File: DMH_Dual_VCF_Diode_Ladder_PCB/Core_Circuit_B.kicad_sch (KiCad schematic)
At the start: 41 parts, among them SW4 SW_SPDT, SW5 SW_SPDT, SW6 SW_SPDT, U4 TL074, U6 TL074

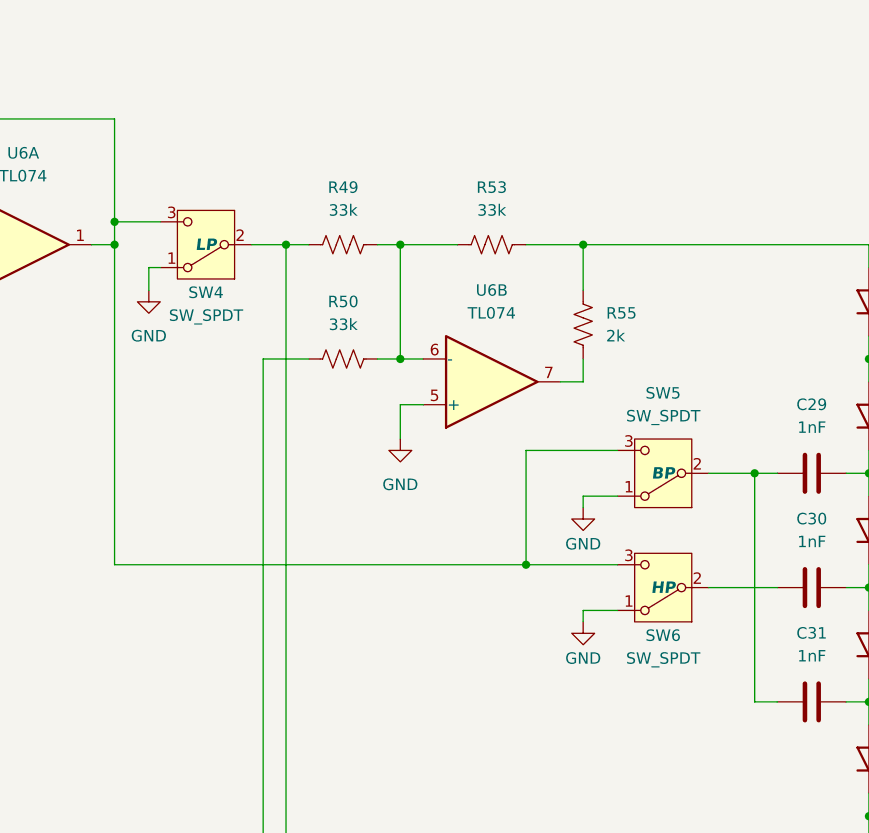
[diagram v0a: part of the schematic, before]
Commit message: Finished routing
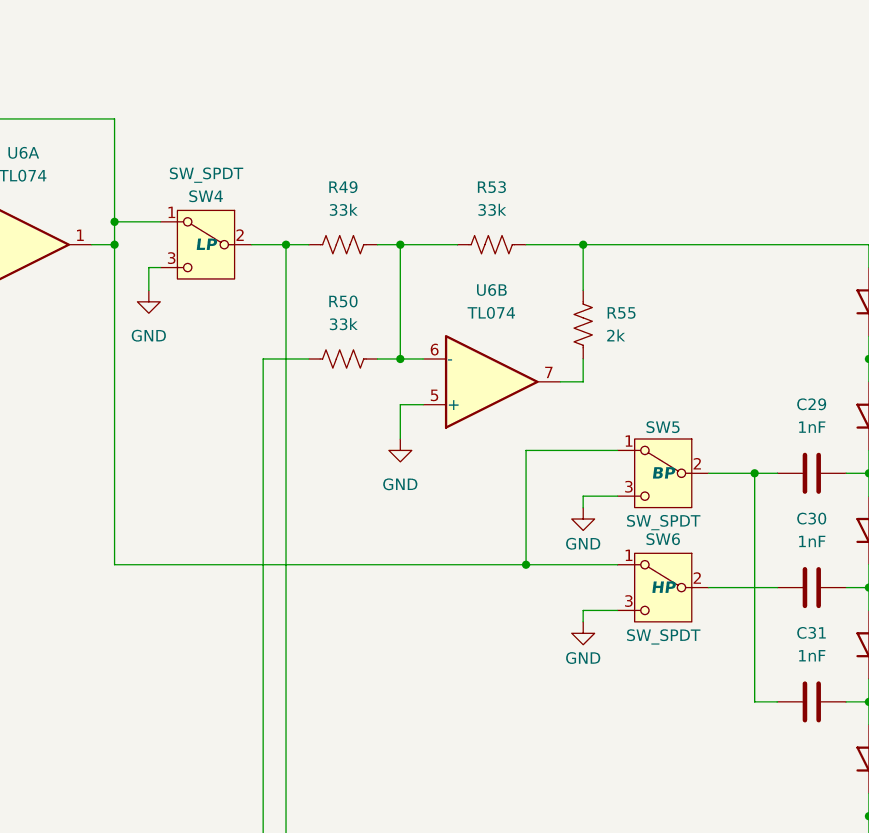
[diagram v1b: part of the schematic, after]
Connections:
- net GND: now also SW4.3 (C), SW5.3 (C), SW6.3 (C); no longer SW4.1 (A), SW5.1 (A), SW6.1 (A)
- new net: SW4.1 (A), SW5.1 (A), SW6.1 (A), U6.1, U6.2 (-)
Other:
- moved on the sheet: SW4, SW5, SW6
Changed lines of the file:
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@@
 	(symbol
 		(lib_id "Switch:SW_SPDT")
-		(at 135.89 86.36 180)
-		(unit 1)
-		(exclude_from_sim no)
-		(in_bom yes)
-		(on_board yes)
-		(dnp no)
-		(fields_autoplaced yes)
+		(at 135.89 86.36 0)
+		(mirror y)
+		(unit 1)
+		(exclude_from_sim no)
+		(in_bom yes)
+		(on_board yes)
+		(dnp no)
 		(property "Reference" "SW5"
-			(at 135.89 77.47 0)
+			(at 135.89 81.28 0)
 			(effects
 				(font
@@
 		)
 		(property "Value" "SW_SPDT"
-			(at 135.89 80.01 0)
+			(at 135.89 91.694 0)
 			(effects
 				(font
@@
 		)
 		(property "Datasheet" "~"
-			(at 135.89 78.74 0)
+			(at 135.89 93.98 0)
 			(effects
 				(font
@@
 	(symbol
 		(lib_id "Switch:SW_SPDT")
-		(at 135.89 99.06 180)
+		(at 135.89 99.06 0)
+		(mirror y)
 		(unit 1)
 		(exclude_from_sim no)
@@
 		(dnp no)
 		(property "Reference" "SW6"
+			(at 135.89 93.726 0)
+			(effects
+				(font
+					(size 1.27 1.27)
+				)
+			)
+		)
+		(property "Value" "SW_SPDT"
 			(at 135.89 104.394 0)
-			(effects
-				(font
-					(size 1.27 1.27)
-				)
-			)
-		)
-		(property "Value" "SW_SPDT"
-			(at 135.89 106.934 0)
 			(effects
 				(font
@@
 		)
 		(property "Datasheet" "~"
-			(at 135.89 91.44 0)
+			(at 135.89 106.68 0)
 			(effects
 				(font
@@
 	(symbol
 		(lib_id "Switch:SW_SPDT")
-		(at 85.09 60.96 180)
+		(at 85.09 60.96 0)
+		(mirror y)
 		(unit 1)
 		(exclude_from_sim no)
@@
 		(dnp no)
 		(property "Reference" "SW4"
-			(at 85.09 66.294 0)
+			(at 85.09 55.626 0)
 			(effects
 				(font
@@
 		)
 		(property "Value" "SW_SPDT"
-			(at 85.09 68.834 0)
+			(at 85.09 53.086 0)
 			(effects
 				(font
@@
 		)
 		(property "Datasheet" "~"
-			(at 85.09 53.34 0)
-			(effects
-				(font
+			(at 85.09 68.58 0)
+			(effects
+				(font
